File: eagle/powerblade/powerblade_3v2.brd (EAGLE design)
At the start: 25.4 x 25.4 mm, 79 parts, among them J1 JTAG_14PIN_IDC-ND, J2 AC_INF4, J4 TC2030-JLINK-NL, Q1 NTS4173, Q4 2SK1829, U1 TPS62122, U2 MCP6V3, U3 MSP430FR5738, U4 NRF51822QF, U6 MAX9910, U7 OPA2369, X1 16MHz, X3 32.768kHz, Y1 UREACH_XTEND

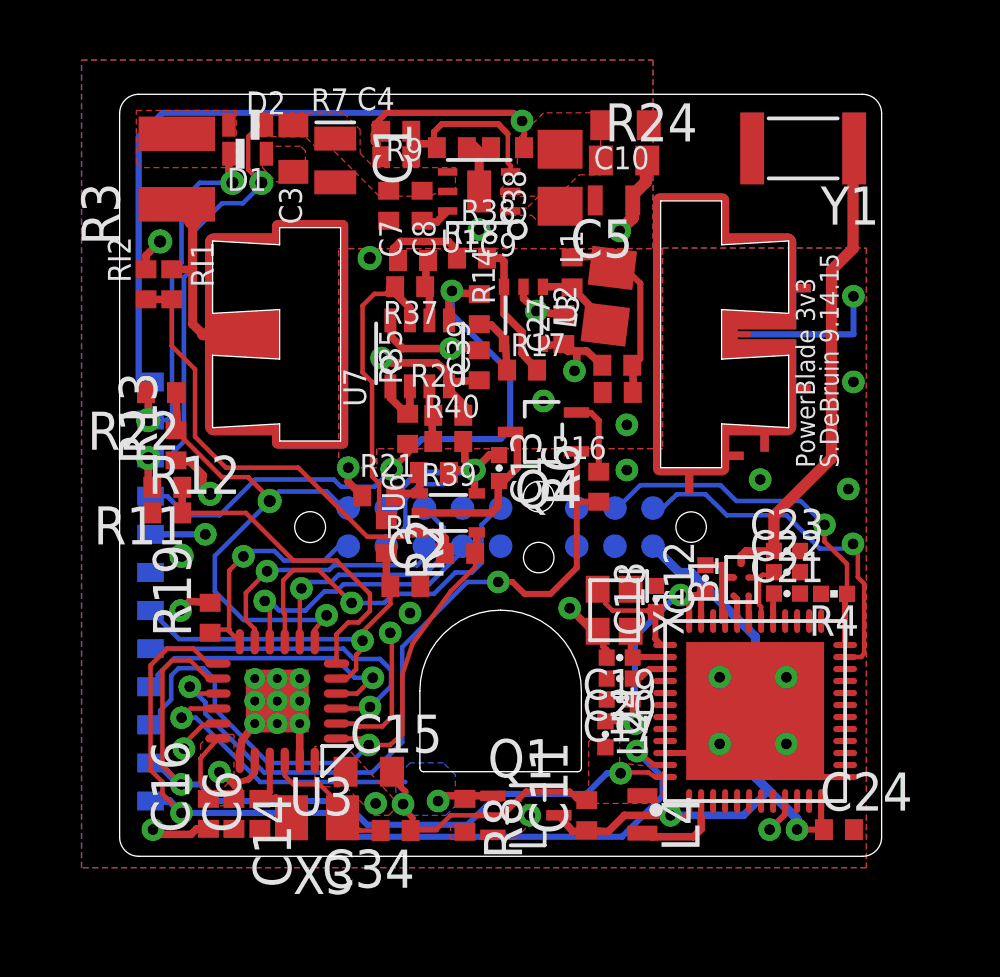
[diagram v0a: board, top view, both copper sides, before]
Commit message: updated l41
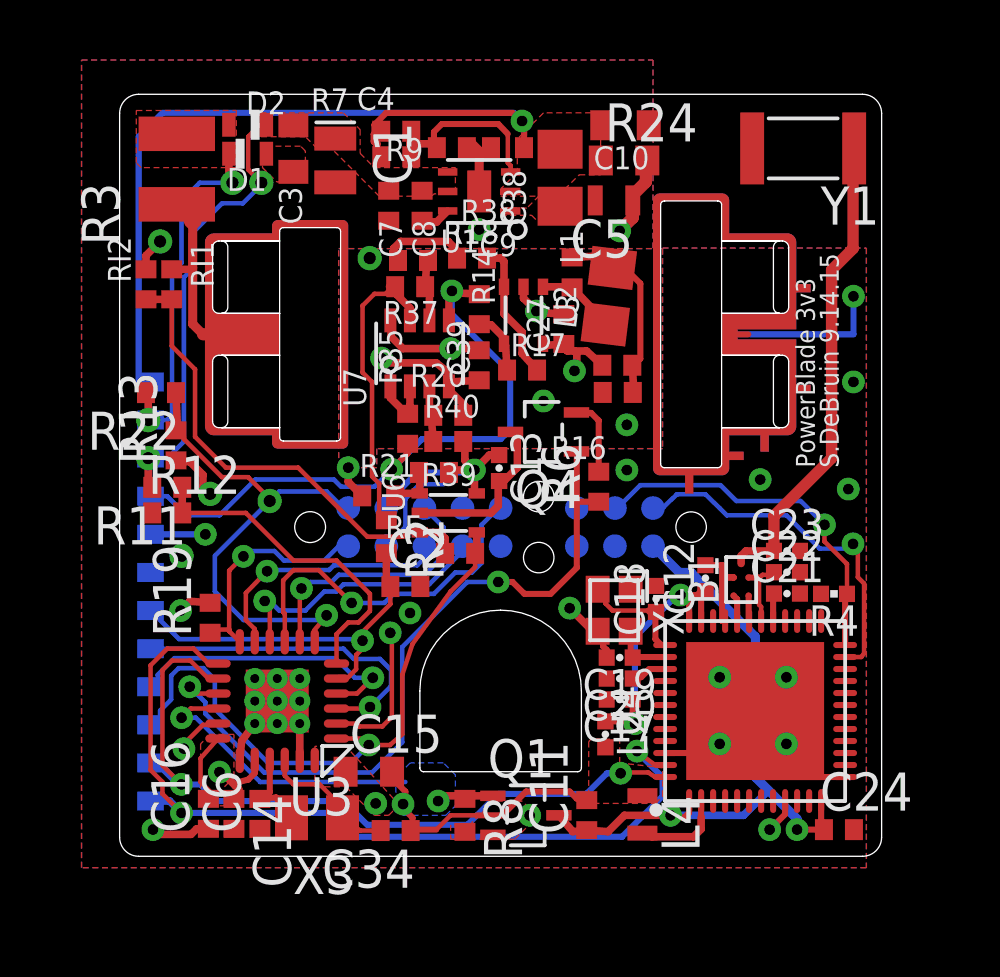
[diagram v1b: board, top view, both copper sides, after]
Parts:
- J2: value AC_INF4 -> AC_INF41; device powerfilm:AC3_F4 -> powerfilm:AC3_F41
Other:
- outline, holes or cut-outs redrawn
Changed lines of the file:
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@@
 <?xml version="1.0" encoding="utf-8"?>
 <!DOCTYPE eagle SYSTEM "eagle.dtd">
-<eagle version="6.5.0">
+<eagle version="6.3">
 <drawing>
 <settings>
@@
 <attribute name="DIGIKEY" value="490-4025-1-ND" x="4.727575" y="-16.002" size="1.778" layer="27" rot="R270" display="off"/>
 </element>
-<element name="J2" library="powerfilm" package="AC3_F4" value="AC_INF4" x="0" y="0">
+<element name="J2" library="powerfilm" package="AC3_F41" value="AC_INF41" x="0" y="0">
 <attribute name="DIGIKEY" value="ED1649-ND" x="0" y="0" size="1.778" layer="27" display="off"/>
 <attribute name="DIGIKEY_2" value="ED1649-ND" x="0" y="0" size="1.778" layer="27" display="off"/>
@@
 </signal>
 </signals>
-<errors>
-</errors>
 </board>
 </drawing>
